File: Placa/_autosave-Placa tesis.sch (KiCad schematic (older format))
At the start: 78 parts, among them J1 OKI-78SR, J10 Conn_01x01, J11 USB_B_Micro, J12 Conn_01x01, J13 Conn_01x05, J14 INA226, J15 Conn_01x04, J2 Conn_01x04, J3 FUENTE, J4 DHT11, J5 COMM, J6 Conn_01x08, J7 Conn_01x11, J8 Conn_01x11, J9 Conn_01x03, Q1 Q_NMOS_GDS, Q2 Q_NMOS_GDS, Q3 Q_NMOS_GDS, Q4 Q_NMOS_GDS, SW1 SW_Push, SW2 SW_Push, U2 Nodemcuv_3, U3 INA226, U4 LM3464AMH_NOPB, U5 ESP-12E, U6 ESP-12E, U9 FT230XS

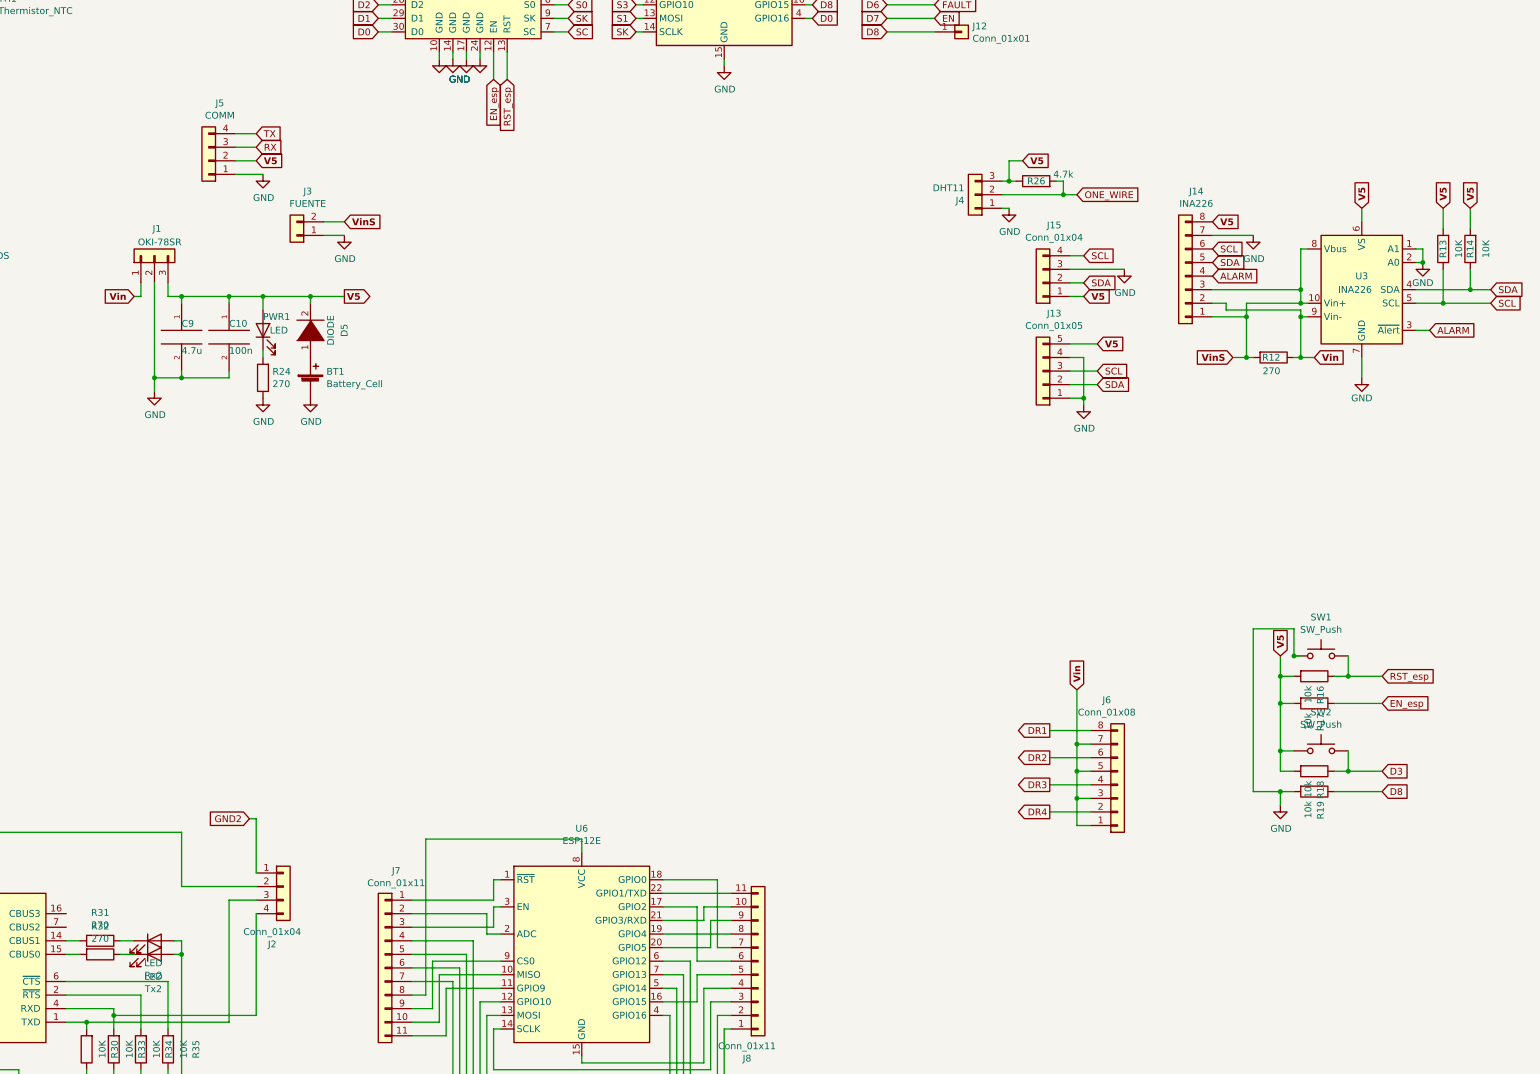
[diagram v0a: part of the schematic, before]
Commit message: La venganza
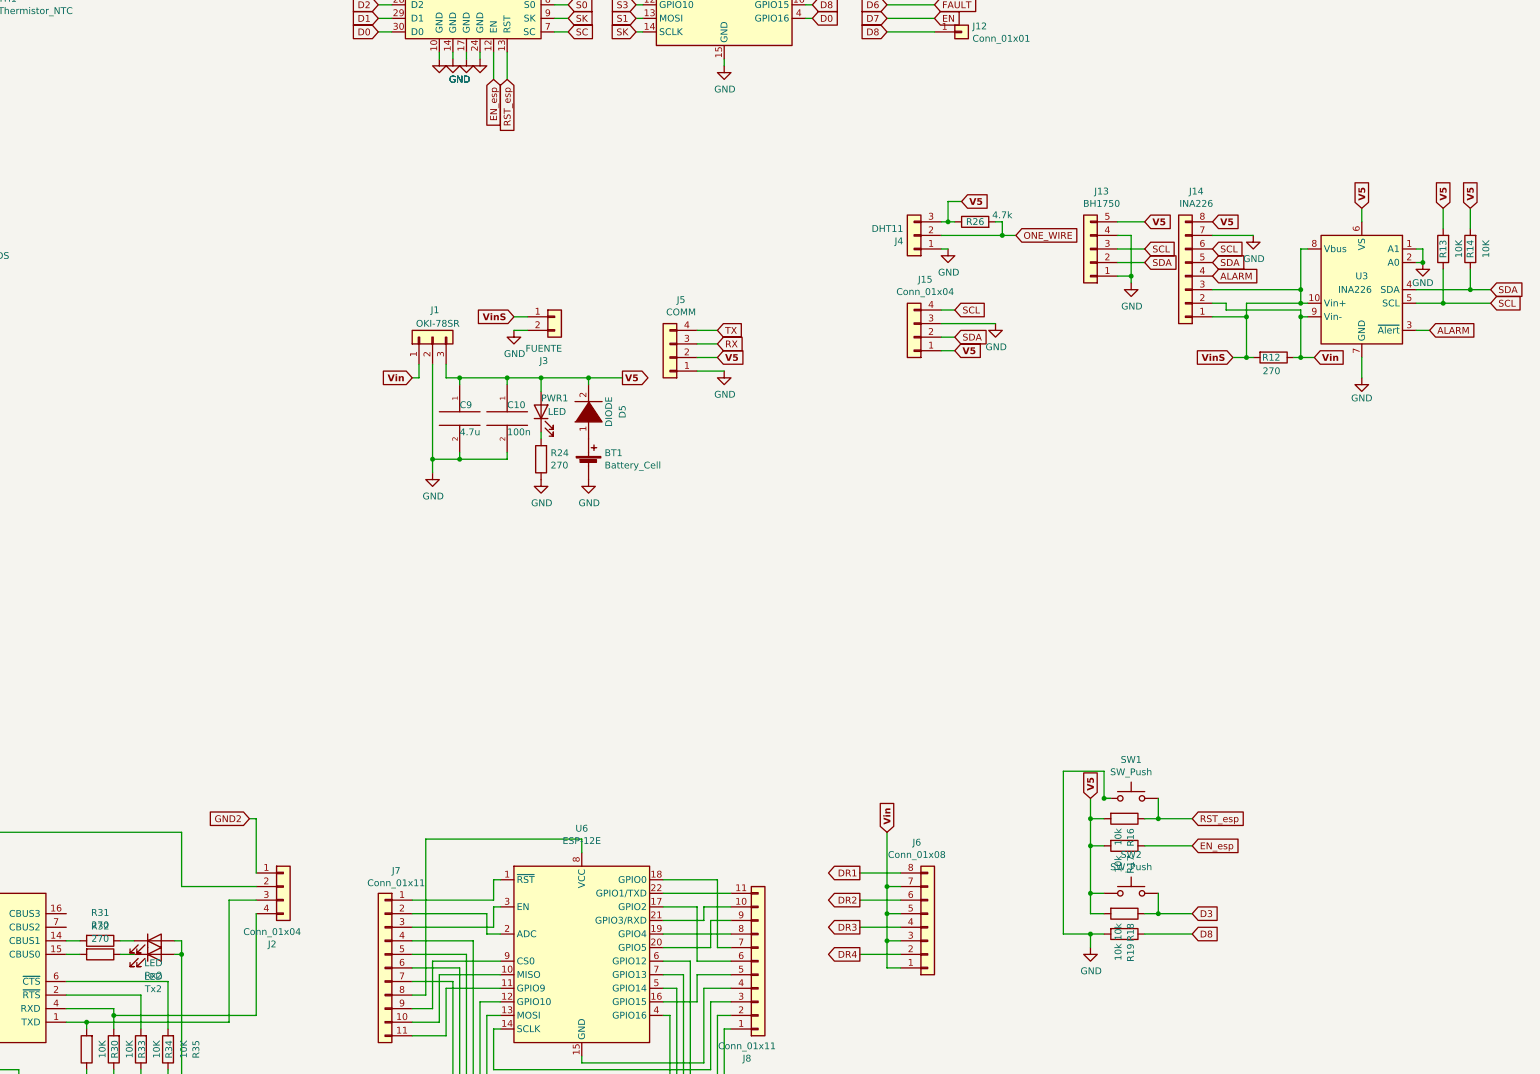
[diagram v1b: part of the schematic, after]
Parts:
- J13: value Conn_01x05 -> BH1750
- U4: footprint LM3464AMH_NOPB:SOP65P640X110-29N -> USERPKG:IC_TPS61196PWPRQ1
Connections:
- net GND: now also J3.2 (Pin_2); no longer J3.1 (Pin_1)
- net VinS: now also J3.1 (Pin_1); no longer J3.2 (Pin_2)
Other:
- moved on the sheet: BT1, C10, C9, D5, J1, J13, J15, J3, J4, J5, J6, PWR1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
